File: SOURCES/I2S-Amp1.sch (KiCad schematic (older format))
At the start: 34 parts, among them P10 CONN_01X02, P17 TST, P9 CONN_01X02, U3 SN74LVC14ADG4, U4 TAS5760MDCAR

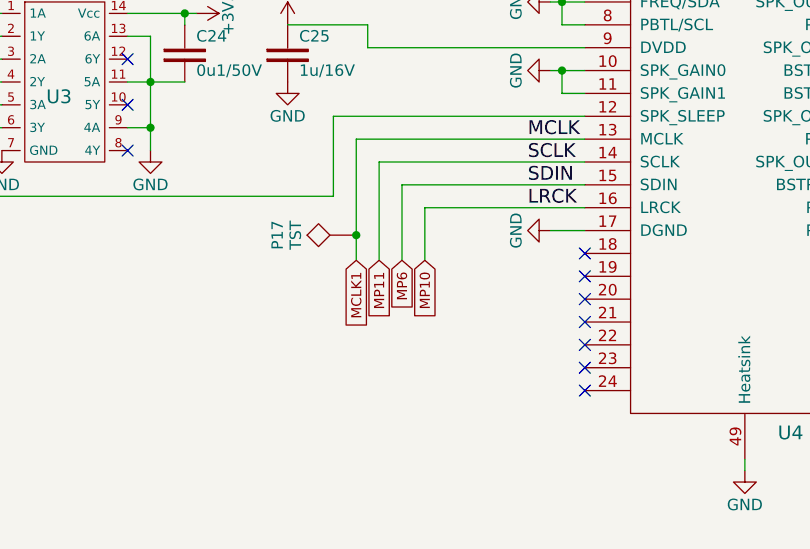
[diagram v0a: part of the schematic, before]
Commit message: started layout
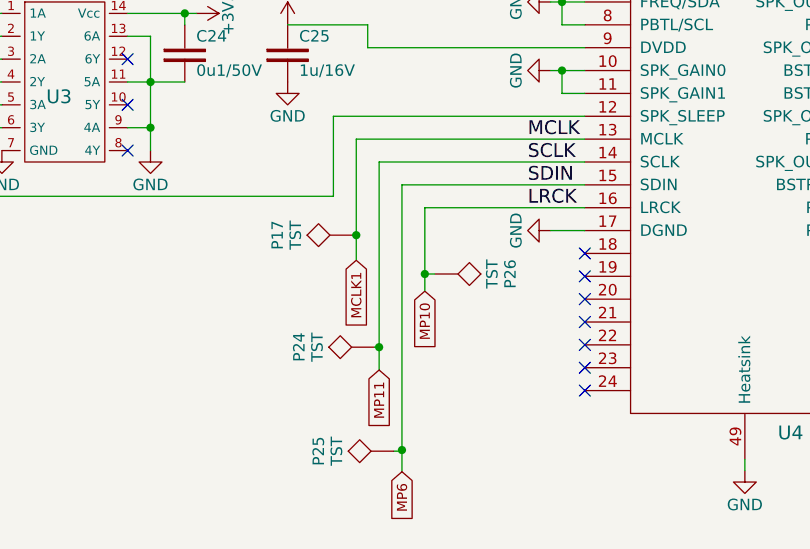
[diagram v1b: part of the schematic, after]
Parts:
- added P24, P25, P26: TST, fdsp_misc:Measurement_Point_Round-SMD-Pad_Small, symbol TST
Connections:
- net MP10: now also P26.1
- net MP11: now also P24.1
- net MP6: now also P25.1
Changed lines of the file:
@@
 	4050 3100 4050 3630
 Wire Wire Line
-	4150 3200 4150 3630
+	4150 3200 4150 4110
 Wire Wire Line
-	4250 3300 4250 3630
+	4250 3300 4250 4555
 Wire Wire Line
-	4350 3400 4350 3630
+	4350 3400 4350 3765
 $Comp
 L +3V3 #PWR063
@@
 	1    0    0    -1
 $EndComp
-Text GLabel 4350 3630 3    44   Input ~ 0
+Text GLabel 4350 3765 3    44   Input ~ 0
 MP10
-Text GLabel 4250 3630 3    44   Input ~ 0
+Text GLabel 4250 4555 3    44   Input ~ 0
 MP6
-Text GLabel 4150 3630 3    44   Input ~ 0
+Text GLabel 4150 4110 3    44   Input ~ 0
 MP11
 Text GLabel 4050 3630 3    44   Input ~ 0
@@
 	4035 3520 4050 3520
 Connection ~ 4050 3520
+$Comp
+L TST P24
+U 1 1 5B23E70D
+P 4130 4010
+F 0 "P24" H 4130 4310 50  0000 C BNN
+F 1 "TST" H 4130 4260 50  0000 C CNN
+F 2 "fdsp_misc:Measurement_Point_Round-SMD-Pad_Small" H 4130 4010 50  0001 C CNN
+F 3 "" H 4130 4010 50  0000 C CNN
+	1    4130 4010
+	0    -1   -1   0
+$EndComp
+Wire Wire Line
+	4130 4010 4150 4010
+Connection ~ 4150 4010
+$Comp
+L TST P25
+U 1 1 5B23EE58
+P 4215 4465
+F 0 "P25" H 4215 4765 50  0000 C BNN
+F 1 "TST" H 4215 4715 50  0000 C CNN
+F 2 "fdsp_misc:Measurement_Point_Round-SMD-Pad_Small" H 4215 4465 50  0001 C CNN
+F 3 "" H 4215 4465 50  0000 C CNN
+	1    4215 4465
+	0    -1   -1   0
+$EndComp
+Wire Wire Line
+	4215 4465 4250 4465
+Wire Wire Line
+	4250 4465 4250 4460
+Connection ~ 4250 4460
+$Comp
+L TST P26
+U 1 1 5B23F295
+P 4395 3690
+F 0 "P26" H 4395 3990 50  0000 C BNN
+F 1 "TST" H 4395 3940 50  0000 C CNN
+F 2 "fdsp_misc:Measurement_Point_Round-SMD-Pad_Small" H 4395 3690 50  0001 C CNN
+F 3 "" H 4395 3690 50  0000 C CNN
+	1    4395 3690
+	0    1    1    0
+$EndComp
+Wire Wire Line
+	4395 3690 4350 3690
+Connection ~ 4350 3690
 $EndSCHEMATC
